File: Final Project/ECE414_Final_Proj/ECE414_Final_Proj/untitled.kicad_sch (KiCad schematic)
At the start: 39 parts, among them J2 AudioJack2_SwitchT, SW2 SW_Push, SW4 SW_Push_Clockwise, U1 TXS0108EPW, U10 RPi Pico, U11 74HC595, U12 YM3812, U13 YM3014B, U15 TL072, U2 74HC04, U3B1 TL072, U9 LT1086-ADJ, Y2 3.58MHz

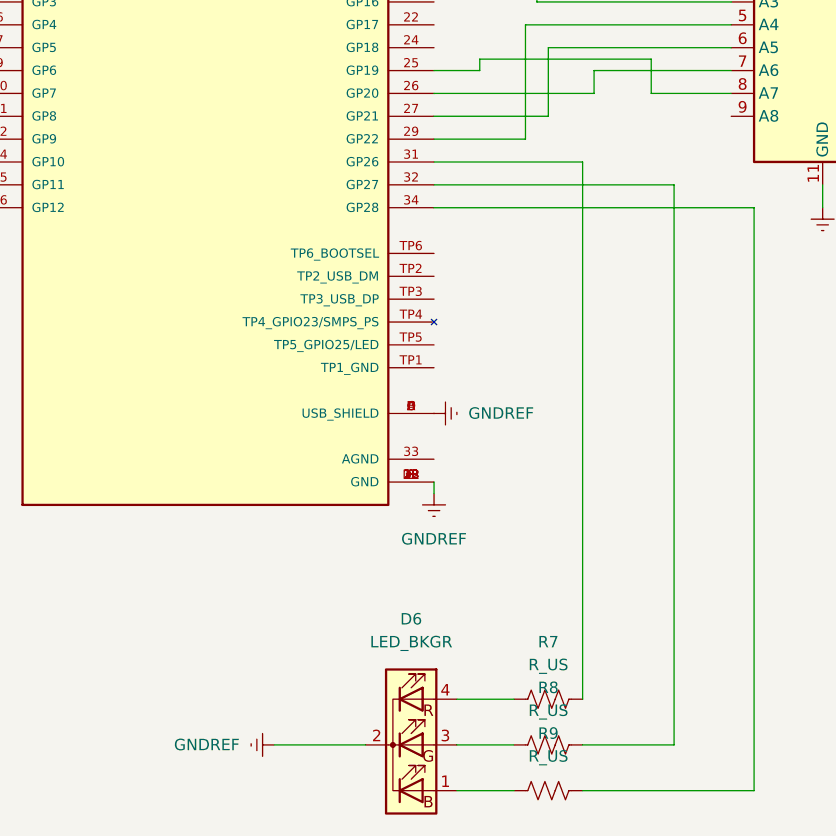
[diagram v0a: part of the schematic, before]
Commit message: Other fixin's
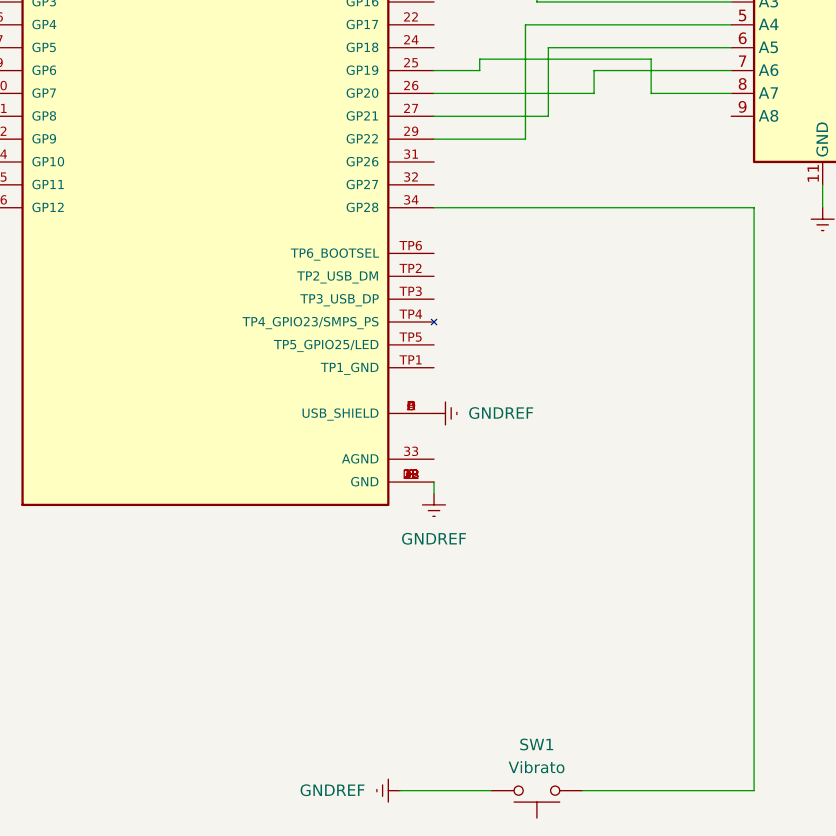
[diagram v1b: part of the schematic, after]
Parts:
- removed D6: LED_BKGR, symbol Device:LED_BKGR
- removed R7, R8, R9: R_US, symbol Device:R_US
- added SW1: Vibrato, symbol Switch:SW_Push
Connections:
- net GNDREF: now also SW1.2
- net at U10.34 (GP28): now also SW1.1
